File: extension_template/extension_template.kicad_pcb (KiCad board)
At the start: 4 copper layers, 30 x 30 mm, 23 parts, among them IC3 TLV61225DC, J6 MISC

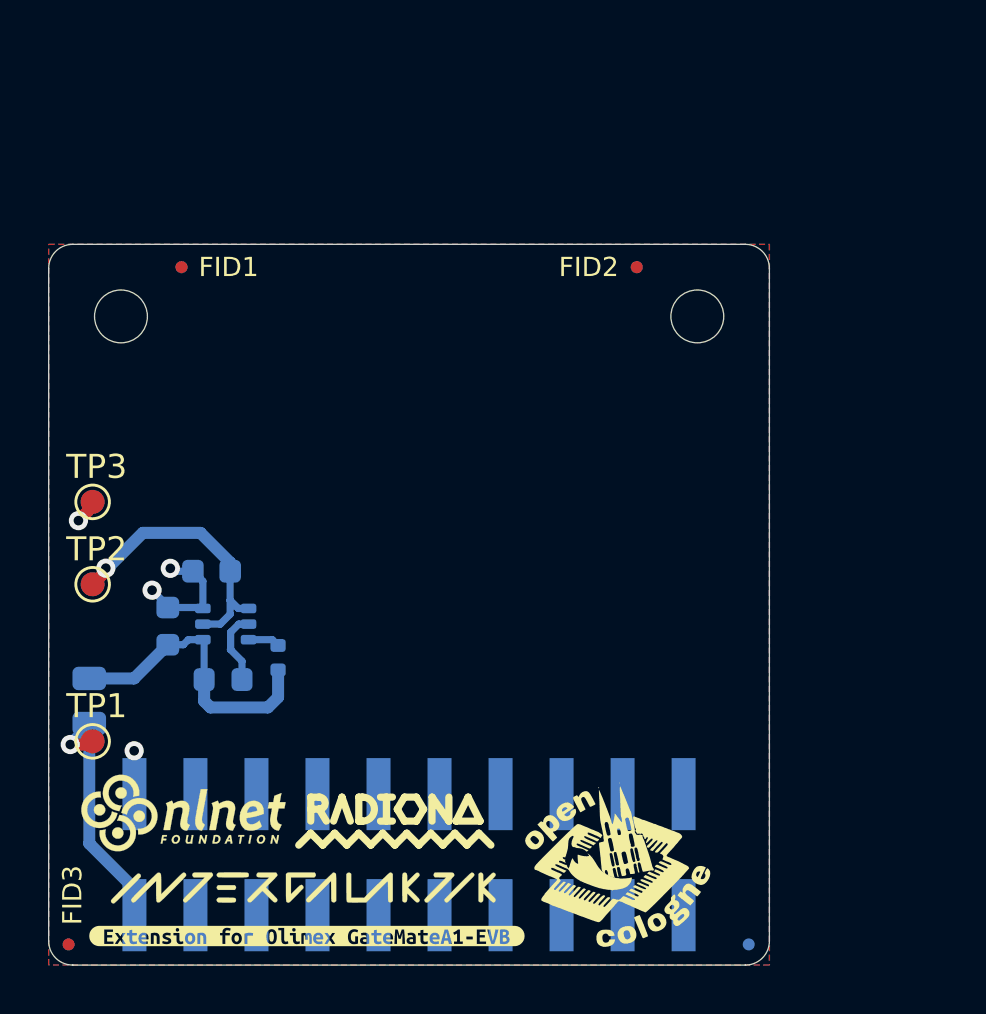
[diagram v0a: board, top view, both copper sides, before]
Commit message: Template update
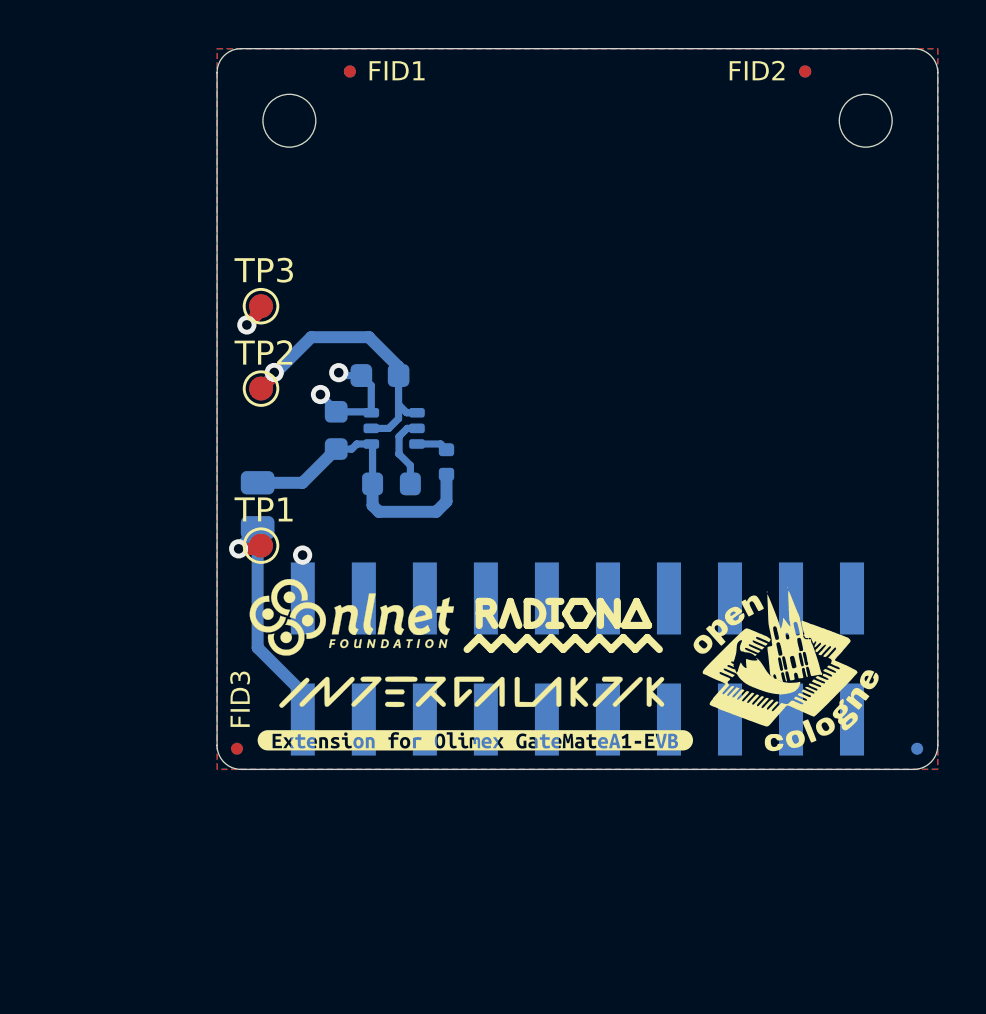
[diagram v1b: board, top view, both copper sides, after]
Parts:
- moved FID3 10.7 mm to (86.1, 81.0)
- moved FID6 10.7 mm to (114.4, 81.0)
- moved H2 10.7 mm to (90.9, 75.5)
- moved J6 10.7 mm to (100.2, 77.2)
- moved TP1 10.7 mm to (87.1, 72.5)
- moved FID1 10.7 mm to (90.8, 52.8)
- moved FID2 10.7 mm to (109.7, 52.8)
- moved FID4 10.7 mm to (109.7, 52.8)
- moved FID5 10.7 mm to (90.8, 52.8)
- moved TP3 10.7 mm to (87.1, 62.6)
- moved C13 10.7 mm to (90.2, 67.7)
- moved C14 10.7 mm to (92.0, 65.4)
- moved H1 10.7 mm to (95.9, 78.5)
- moved H4 10.7 mm to (99.7, 74.8)
- moved H5 10.7 mm to (88.3, 54.8)
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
